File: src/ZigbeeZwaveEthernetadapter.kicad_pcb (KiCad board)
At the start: 2 copper layers, 100 x 100 mm, 1 part

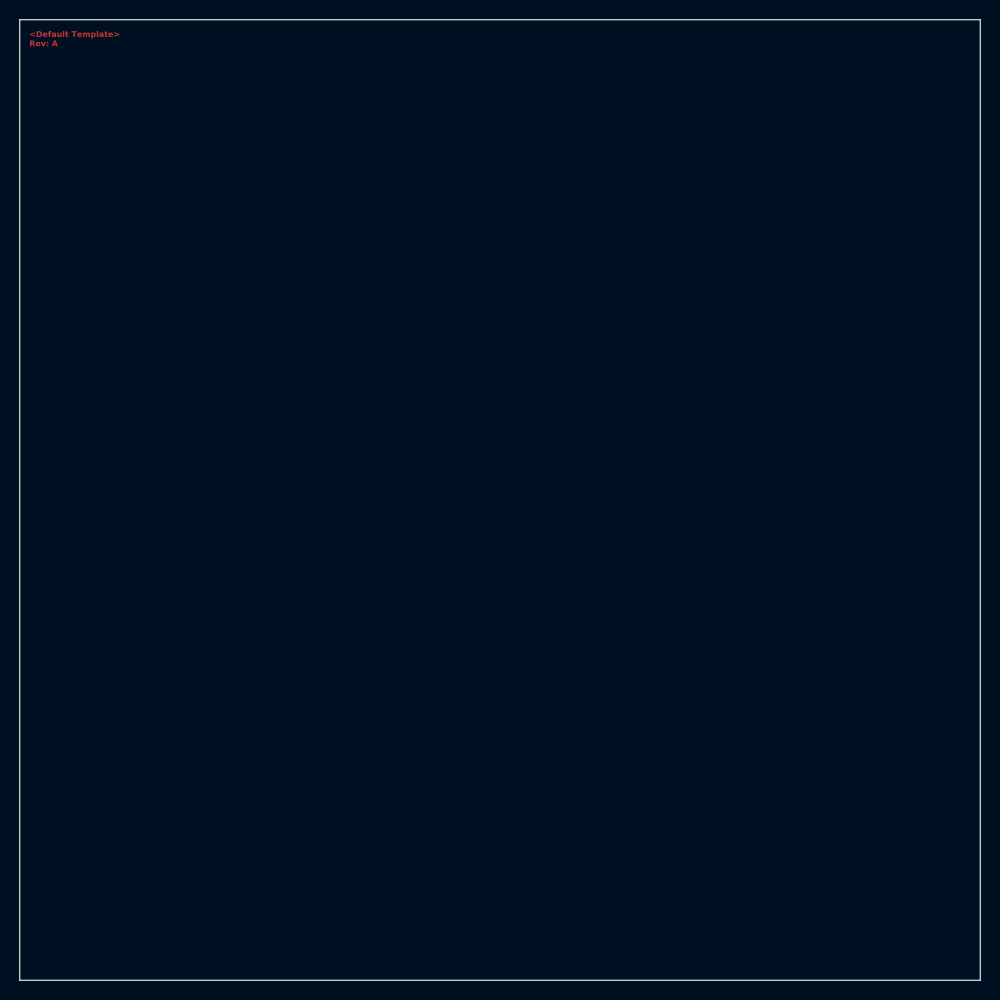
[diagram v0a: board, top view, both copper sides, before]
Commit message: Mod: Schematic and PCB-Layout, finished new Version.
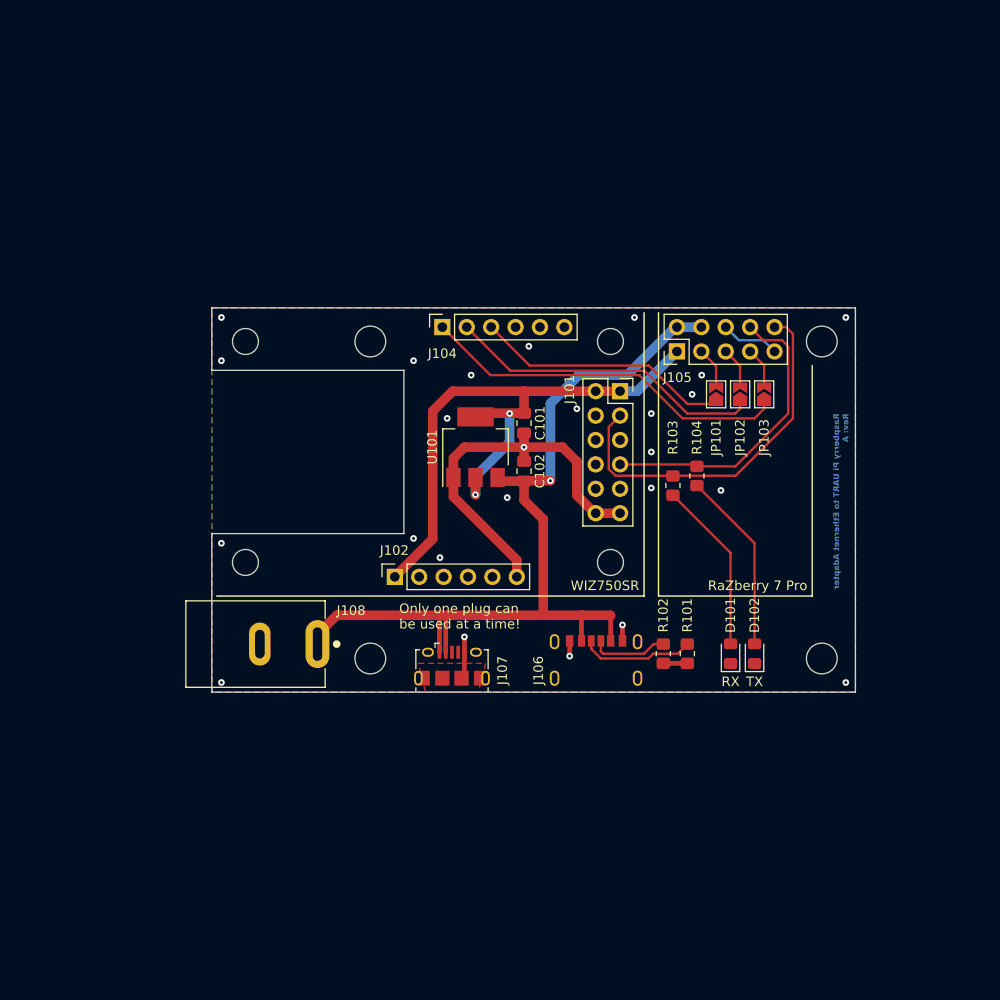
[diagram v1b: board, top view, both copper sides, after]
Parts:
- removed G0: LOGO, drawings:elektronik-emblem_3x3.5_solder
- added C101: 100µF, Capacitor_SMD:C_0805_2012Metric_Pad1.18x1.45mm_HandSolder, F.Cu at (152.5, 82.0)
- added C102: 10µF, Capacitor_SMD:C_0805_2012Metric_Pad1.18x1.45mm_HandSolder, F.Cu at (152.5, 87.0)
- added D101: GN, LED_SMD:LED_0805_2012Metric_Pad1.15x1.40mm_HandSolder, F.Cu at (174.0, 106.0)
- added D102: YE, LED_SMD:LED_0805_2012Metric_Pad1.15x1.40mm_HandSolder, F.Cu at (176.5, 106.0)
- added G***: LOGO, Drawings_User:elektronik-emblem_10x11.6_solder, B.Cu at (175.5, 90.0)
- added H101: MountingHole, MountingHole:MountingHole_2.7mm_M2.5_DIN965, F.Cu at (123.5, 73.5)
- added H102: MountingHole, MountingHole:MountingHole_2.7mm_M2.5_DIN965, F.Cu at (161.5, 73.5)
- added H103: MountingHole, MountingHole:MountingHole_2.7mm_M2.5_DIN965, F.Cu at (161.5, 96.5)
- added H104: MountingHole, MountingHole:MountingHole_2.7mm_M2.5_DIN965, F.Cu at (123.5, 96.5)
- added H105: MountingHole, MountingHole:MountingHole_3.2mm_M3_DIN965, F.Cu at (136.5, 73.5)
- added H106: MountingHole, MountingHole:MountingHole_3.2mm_M3_DIN965, F.Cu at (183.5, 73.5)
- added H107: MountingHole, MountingHole:MountingHole_3.2mm_M3_DIN965, F.Cu at (183.5, 106.5)
- added H108: MountingHole, MountingHole:MountingHole_3.2mm_M3_DIN965, F.Cu at (136.5, 106.5)
- added J101: Conn_02x06_Odd_Even, Connector_PinSocket_2.54mm:PinSocket_2x06_P2.54mm_Vertical, F.Cu at (162.5, 78.7)
- added J102: Conn_01x06, Connector_PinSocket_2.54mm:PinSocket_1x06_P2.54mm_Vertical, F.Cu at (139.1, 98.0)
- added J104: Conn_01x06, Connector_PinSocket_2.54mm:PinSocket_1x06_P2.54mm_Vertical, F.Cu at (144.0, 72.0)
- added J105: Conn_02x05_Odd_Even, Connector_PinHeader_2.54mm:PinHeader_2x05_P2.54mm_Vertical, F.Cu at (168.4, 74.5)
- added J106: USB4125-GF-A, Connector_User:GCT_USB4125-GF-A, F.Cu at (160.0, 107.8)
- added J107: USB_B_Micro, Connector_USB:USB_Micro-B_Amphenol_10118194_Horizontal, F.Cu at (145.0, 107.2)
- added J108: Barrel_Jack, Connector_User:CUI_PJ-037A, F.Cu at (131.0, 105.0)
- added JP101: SolderJumper_2_Open, Jumper:SolderJumper-2_P1.3mm_Open_TrianglePad1.0x1.5mm, F.Cu at (172.5, 79.0)
- added JP102: SolderJumper_2_Open, Jumper:SolderJumper-2_P1.3mm_Open_TrianglePad1.0x1.5mm, F.Cu at (175.0, 79.0)
- added JP103: SolderJumper_2_Open, Jumper:SolderJumper-2_P1.3mm_Open_TrianglePad1.0x1.5mm, F.Cu at (177.5, 79.0)
- added R101: 5.1k, Resistor_SMD:R_0805_2012Metric_Pad1.20x1.40mm_HandSolder, F.Cu at (169.5, 106.0)
- added R102: 5.1k, Resistor_SMD:R_0805_2012Metric_Pad1.20x1.40mm_HandSolder, F.Cu at (167.0, 106.0)
- added R103: 100R, Resistor_SMD:R_0805_2012Metric_Pad1.20x1.40mm_HandSolder, F.Cu at (168.0, 88.5)
- added R104: 100R, Resistor_SMD:R_0805_2012Metric_Pad1.20x1.40mm_HandSolder, F.Cu at (170.5, 87.5)
- added U101: TLV1117-33, Package_TO_SOT_SMD:SOT-223-3_TabPin2, F.Cu at (147.4, 84.5)
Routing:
- net +5V: track 0.00 -> 93.1 mm, vias 0 -> 1
- net +3V3: track 0.00 -> 66.4 mm, vias 0 -> 2
- net GND: track 0.00 -> 57.1 mm, vias 0 -> 25
- net /RXD: track 0.00 -> 39.0 mm
- net /GPIO_D: track 0.00 -> 38.6 mm
- net /GPIO_C: track 0.00 -> 33.2 mm
- net /TXD: track 0.00 -> 31.7 mm
- net /GPIO_B: track 0.00 -> 26.8 mm
- net Net-(D102-A): track 0.00 -> 19.0 mm
- net Net-(D101-A): track 0.00 -> 18.0 mm
- net Net-(J106-CC1): track 0.00 -> 11.9 mm
- net Net-(J106-CC2): track 0.00 -> 8.10 mm
- net /GPIO_2: track 0.00 -> 4.37 mm
- net /GPIO_3: track 0.00 -> 4.36 mm
- net /GPIO_4: track 0.00 -> 4.34 mm
- added copper zone on B.Cu, net GND
- added copper zone on F.Cu, net GND
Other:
- board size 100 x 100 mm -> 67 x 40 mm
- board text added: "Only one plug can be used at a time!"
- board text added: "RX"
- board text added: "RaZberry 7 Pro"
- board text added: "TX"
- board text added: "WIZ750SR"
